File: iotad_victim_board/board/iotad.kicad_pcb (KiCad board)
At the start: 2 copper layers, 27.9 x 27.9 mm, 30 parts, among them P1 CONN_01X10, P2 CONN_01X06, U11 24C16, U2 MAX31820

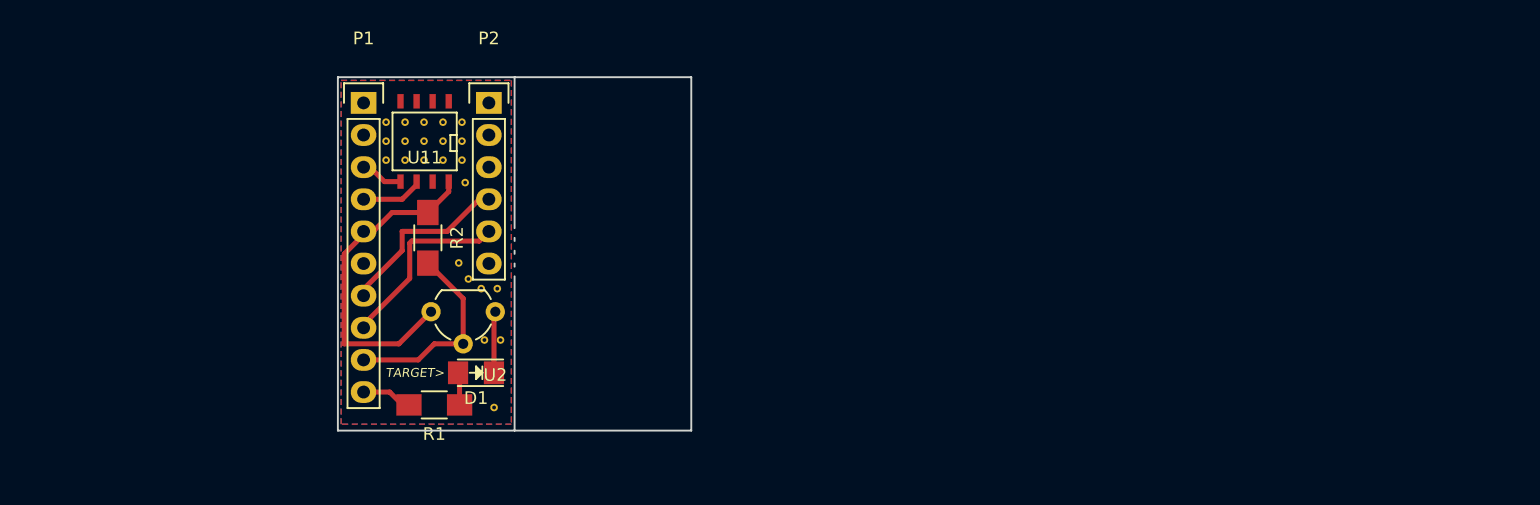
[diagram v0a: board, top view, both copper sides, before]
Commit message: storing
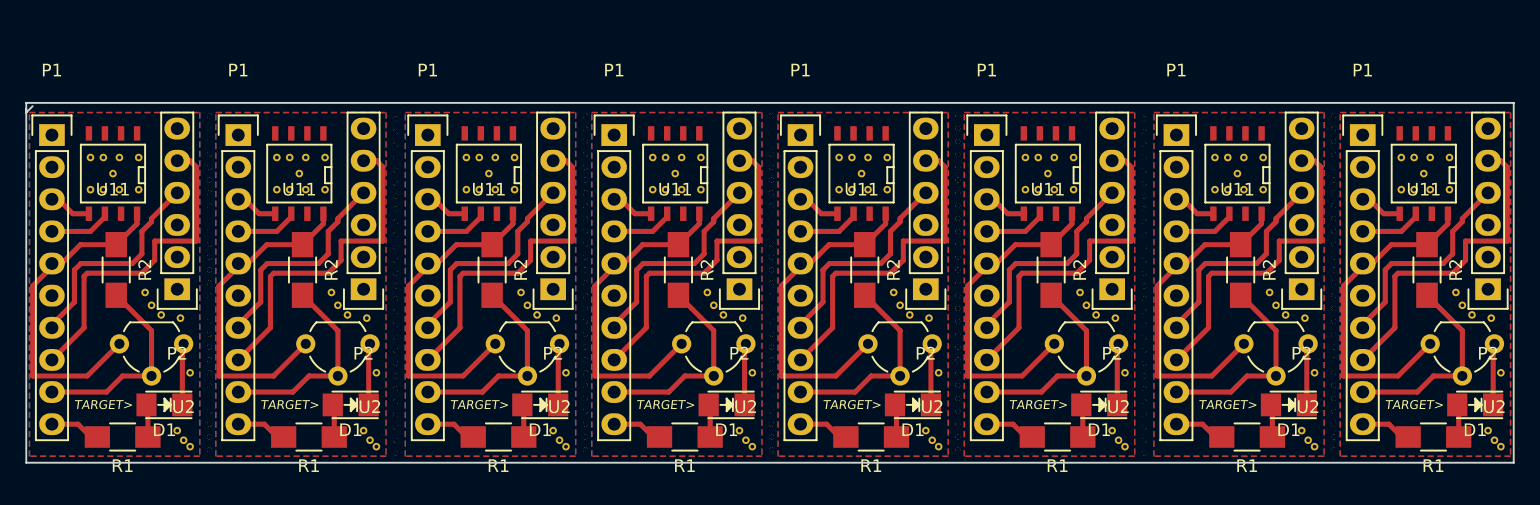
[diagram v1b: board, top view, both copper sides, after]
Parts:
- added D1: LED, LEDs:LED_1206, F.Cu at (182.6, 127.5)
- added D1: LED, LEDs:LED_1206, F.Cu at (197.4, 127.5)
- added D1: LED, LEDs:LED_1206, F.Cu at (227.1, 127.5)
- added D1: LED, LEDs:LED_1206, F.Cu at (212.3, 127.5)
- added D1: LED, LEDs:LED_1206, F.Cu at (153.2, 127.5)
- added D1: LED, LEDs:LED_1206, F.Cu at (167.9, 127.5)
- added D1: LED, LEDs:LED_1206, F.Cu at (138.2, 127.5)
- added P1: CONN_01X10, Pin_Headers:Pin_Header_Straight_1x10, F.Cu at (173.7, 106.2)
- added P1: CONN_01X10, Pin_Headers:Pin_Header_Straight_1x10, F.Cu at (188.5, 106.2)
- added P1: CONN_01X10, Pin_Headers:Pin_Header_Straight_1x10, F.Cu at (218.2, 106.2)
- added P1: CONN_01X10, Pin_Headers:Pin_Header_Straight_1x10, F.Cu at (203.5, 106.2)
- added P1: CONN_01X10, Pin_Headers:Pin_Header_Straight_1x10, F.Cu at (144.3, 106.2)
- added P1: CONN_01X10, Pin_Headers:Pin_Header_Straight_1x10, F.Cu at (159.0, 106.2)
- added P1: CONN_01X10, Pin_Headers:Pin_Header_Straight_1x10, F.Cu at (129.3, 106.2)
- added P2: CONN_01X06, Pin_Headers:Pin_Header_Straight_1x06, F.Cu at (183.6, 118.4)
- added P2: CONN_01X06, Pin_Headers:Pin_Header_Straight_1x06, F.Cu at (198.4, 118.4)
- added P2: CONN_01X06, Pin_Headers:Pin_Header_Straight_1x06, F.Cu at (228.1, 118.4)
- added P2: CONN_01X06, Pin_Headers:Pin_Header_Straight_1x06, F.Cu at (213.4, 118.4)
- added P2: CONN_01X06, Pin_Headers:Pin_Header_Straight_1x06, F.Cu at (154.2, 118.4)
- added P2: CONN_01X06, Pin_Headers:Pin_Header_Straight_1x06, F.Cu at (168.9, 118.4)
- added P2: CONN_01X06, Pin_Headers:Pin_Header_Straight_1x06, F.Cu at (139.2, 118.4)
- added R1: R, Resistors_SMD:R_1206_HandSoldering, F.Cu at (179.3, 130.0)
- added R1: R, Resistors_SMD:R_1206_HandSoldering, F.Cu at (194.1, 130.0)
- added R1: R, Resistors_SMD:R_1206_HandSoldering, F.Cu at (223.8, 130.0)
- added R1: R, Resistors_SMD:R_1206_HandSoldering, F.Cu at (209.0, 130.0)
- added R1: R, Resistors_SMD:R_1206_HandSoldering, F.Cu at (149.9, 130.0)
- added R1: R, Resistors_SMD:R_1206_HandSoldering, F.Cu at (164.6, 130.0)
- added R1: R, Resistors_SMD:R_1206_HandSoldering, F.Cu at (134.9, 130.0)
- added R2: 4.8k, Resistors_SMD:R_1206_HandSoldering, F.Cu at (178.8, 116.8)
- added R2: 4.8k, Resistors_SMD:R_1206_HandSoldering, F.Cu at (193.5, 116.8)
- added R2: 4.8k, Resistors_SMD:R_1206_HandSoldering, F.Cu at (223.3, 116.8)
- added R2: 4.8k, Resistors_SMD:R_1206_HandSoldering, F.Cu at (208.5, 116.8)
- added R2: 4.8k, Resistors_SMD:R_1206_HandSoldering, F.Cu at (149.4, 116.8)
- added R2: 4.8k, Resistors_SMD:R_1206_HandSoldering, F.Cu at (164.1, 116.8)
- added R2: 4.8k, Resistors_SMD:R_1206_HandSoldering, F.Cu at (134.4, 116.8)
- added REF** (x4): DRILL-0.6mm, via-0:DRILL-0.6mm, F.Cu at (186.2, 107.7)
- added REF** (x4): DRILL-0.6mm, via-0:DRILL-0.6mm, F.Cu at (186.2, 104.6)
- added REF** (x4): DRILL-0.6mm, via-0:DRILL-0.6mm, F.Cu at (186.2, 121.9)
- added REF** (x4): DRILL-0.6mm, via-0:DRILL-0.6mm, F.Cu at (186.2, 124.0)
- added REF** (x4): DRILL-0.6mm, via-0:DRILL-0.6mm, F.Cu at (186.2, 122.9)
- added REF** (x4): DRILL-0.6mm, via-0:DRILL-0.6mm, F.Cu at (215.9, 124.0)
- added REF** (x4): DRILL-0.6mm, via-0:DRILL-0.6mm, F.Cu at (215.9, 122.9)
- added REF** (x4): DRILL-0.6mm, via-0:DRILL-0.6mm, F.Cu at (215.9, 121.9)
- added REF** (x4): DRILL-0.6mm, via-0:DRILL-0.6mm, F.Cu at (215.9, 120.9)
- added REF** (x4): DRILL-0.6mm, via-0:DRILL-0.6mm, F.Cu at (186.2, 105.7)
- added REF** (x4): DRILL-0.6mm, via-0:DRILL-0.6mm, F.Cu at (215.9, 126.0)
- added REF** (x4): DRILL-0.6mm, via-0:DRILL-0.6mm, F.Cu at (215.9, 125.0)
- added REF** (x4): DRILL-0.6mm, via-0:DRILL-0.6mm, F.Cu at (215.9, 128.0)
- added REF** (x4): DRILL-0.6mm, via-0:DRILL-0.6mm, F.Cu at (215.9, 127.0)
- added REF** (x4): DRILL-0.6mm, via-0:DRILL-0.6mm, F.Cu at (215.9, 130.0)
- added REF** (x4): DRILL-0.6mm, via-0:DRILL-0.6mm, F.Cu at (215.9, 129.0)
- added REF** (x4): DRILL-0.6mm, via-0:DRILL-0.6mm, F.Cu at (215.9, 131.1)
- added REF** (x4): DRILL-0.6mm, via-0:DRILL-0.6mm, F.Cu at (215.9, 115.8)
- added REF** (x4): DRILL-0.6mm, via-0:DRILL-0.6mm, F.Cu at (215.9, 114.8)
- added REF** (x4): DRILL-0.6mm, via-0:DRILL-0.6mm, F.Cu at (215.9, 113.8)
- added REF** (x4): DRILL-0.6mm, via-0:DRILL-0.6mm, F.Cu at (215.9, 112.8)
- added REF** (x4): DRILL-0.6mm, via-0:DRILL-0.6mm, F.Cu at (215.9, 117.9)
- added REF** (x4): DRILL-0.6mm, via-0:DRILL-0.6mm, F.Cu at (186.2, 109.7)
- added REF** (x4): DRILL-0.6mm, via-0:DRILL-0.6mm, F.Cu at (215.9, 116.8)
- added REF** (x4): DRILL-0.6mm, via-0:DRILL-0.6mm, F.Cu at (215.9, 119.9)
- added REF** (x4): DRILL-0.6mm, via-0:DRILL-0.6mm, F.Cu at (215.9, 118.9)
- added REF** (x4): DRILL-0.6mm, via-0:DRILL-0.6mm, F.Cu at (186.2, 108.7)
- added REF** (x4): DRILL-0.6mm, via-0:DRILL-0.6mm, F.Cu at (215.9, 111.8)
- added REF** (x4): DRILL-0.6mm, via-0:DRILL-0.6mm, F.Cu at (215.9, 110.7)
- added REF** (x4): DRILL-0.6mm, via-0:DRILL-0.6mm, F.Cu at (215.9, 109.7)
- added REF** (x4): DRILL-0.6mm, via-0:DRILL-0.6mm, F.Cu at (215.9, 108.7)
- added REF** (x4): DRILL-0.6mm, via-0:DRILL-0.6mm, F.Cu at (186.2, 106.7)
- added REF** (x4): DRILL-0.6mm, via-0:DRILL-0.6mm, F.Cu at (215.9, 105.7)
- added REF** (x4): DRILL-0.6mm, via-0:DRILL-0.6mm, F.Cu at (215.9, 104.6)
- added REF** (x4): DRILL-0.6mm, via-0:DRILL-0.6mm, F.Cu at (215.9, 107.7)
- added REF** (x4): DRILL-0.6mm, via-0:DRILL-0.6mm, F.Cu at (215.9, 106.7)
- added REF** (x4): DRILL-0.6mm, via-0:DRILL-0.6mm, F.Cu at (200.9, 124.2)
- added REF** (x4): DRILL-0.6mm, via-0:DRILL-0.6mm, F.Cu at (200.9, 123.2)
- added REF** (x4): DRILL-0.6mm, via-0:DRILL-0.6mm, F.Cu at (200.9, 122.2)
- added REF** (x4): DRILL-0.6mm, via-0:DRILL-0.6mm, F.Cu at (200.9, 121.2)
- added REF** (x4): DRILL-0.6mm, via-0:DRILL-0.6mm, F.Cu at (200.9, 126.2)
- added REF** (x4): DRILL-0.6mm, via-0:DRILL-0.6mm, F.Cu at (200.9, 125.2)
- added REF** (x4): DRILL-0.6mm, via-0:DRILL-0.6mm, F.Cu at (200.9, 128.3)
- added REF** (x4): DRILL-0.6mm, via-0:DRILL-0.6mm, F.Cu at (200.9, 127.3)
- added REF** (x4): DRILL-0.6mm, via-0:DRILL-0.6mm, F.Cu at (200.9, 130.3)
- added REF** (x4): DRILL-0.6mm, via-0:DRILL-0.6mm, F.Cu at (186.2, 111.8)
- added REF** (x4): DRILL-0.6mm, via-0:DRILL-0.6mm, F.Cu at (200.9, 129.3)
- added REF** (x4): DRILL-0.6mm, via-0:DRILL-0.6mm, F.Cu at (200.9, 131.3)
- added REF** (x4): DRILL-0.6mm, via-0:DRILL-0.6mm, F.Cu at (186.2, 110.7)
- added REF** (x4): DRILL-0.6mm, via-0:DRILL-0.6mm, F.Cu at (200.9, 116.1)
- added REF** (x4): DRILL-0.6mm, via-0:DRILL-0.6mm, F.Cu at (200.9, 115.1)
- added REF** (x4): DRILL-0.6mm, via-0:DRILL-0.6mm, F.Cu at (200.9, 114.0)
- added REF** (x4): DRILL-0.6mm, via-0:DRILL-0.6mm, F.Cu at (200.9, 113.0)
- added REF** (x4): DRILL-0.6mm, via-0:DRILL-0.6mm, F.Cu at (200.9, 118.1)
- added REF** (x4): DRILL-0.6mm, via-0:DRILL-0.6mm, F.Cu at (200.9, 117.1)
- added REF** (x4): DRILL-0.6mm, via-0:DRILL-0.6mm, F.Cu at (200.9, 120.1)
- added REF** (x4): DRILL-0.6mm, via-0:DRILL-0.6mm, F.Cu at (200.9, 119.1)
- added REF** (x4): DRILL-0.6mm, via-0:DRILL-0.6mm, F.Cu at (200.9, 112.0)
- added REF** (x4): DRILL-0.6mm, via-0:DRILL-0.6mm, F.Cu at (200.9, 111.0)
- added REF** (x4): DRILL-0.6mm, via-0:DRILL-0.6mm, F.Cu at (200.9, 110.0)
- added REF** (x4): DRILL-0.6mm, via-0:DRILL-0.6mm, F.Cu at (200.9, 109.0)
- added REF** (x4): DRILL-0.6mm, via-0:DRILL-0.6mm, F.Cu at (200.9, 105.9)
- added REF** (x4): DRILL-0.6mm, via-0:DRILL-0.6mm, F.Cu at (200.9, 104.9)
- added REF** (x4): DRILL-0.6mm, via-0:DRILL-0.6mm, F.Cu at (200.9, 108.0)
- added REF** (x4): DRILL-0.6mm, via-0:DRILL-0.6mm, F.Cu at (200.9, 106.9)
- added REF** (x4): DRILL-0.6mm, via-0:DRILL-0.6mm, F.Cu at (141.7, 108.0)
- added REF** (x4): DRILL-0.6mm, via-0:DRILL-0.6mm, F.Cu at (141.7, 106.9)
- added REF** (x4): DRILL-0.6mm, via-0:DRILL-0.6mm, F.Cu at (186.2, 119.9)
- added REF** (x4): DRILL-0.6mm, via-0:DRILL-0.6mm, F.Cu at (141.7, 105.9)
- added REF** (x4): DRILL-0.6mm, via-0:DRILL-0.6mm, F.Cu at (141.7, 104.9)
- added REF** (x4): DRILL-0.6mm, via-0:DRILL-0.6mm, F.Cu at (186.2, 118.9)
- added REF** (x4): DRILL-0.6mm, via-0:DRILL-0.6mm, F.Cu at (141.7, 110.0)
- added REF** (x4): DRILL-0.6mm, via-0:DRILL-0.6mm, F.Cu at (141.7, 109.0)
- added REF** (x4): DRILL-0.6mm, via-0:DRILL-0.6mm, F.Cu at (141.7, 112.0)
- added REF** (x4): DRILL-0.6mm, via-0:DRILL-0.6mm, F.Cu at (141.7, 111.0)
- added REF** (x4): DRILL-0.6mm, via-0:DRILL-0.6mm, F.Cu at (141.7, 120.1)
- added REF** (x4): DRILL-0.6mm, via-0:DRILL-0.6mm, F.Cu at (141.7, 119.1)
- added REF** (x4): DRILL-0.6mm, via-0:DRILL-0.6mm, F.Cu at (141.7, 118.1)
- added REF** (x4): DRILL-0.6mm, via-0:DRILL-0.6mm, F.Cu at (141.7, 117.1)
- added REF** (x4): DRILL-0.6mm, via-0:DRILL-0.6mm, F.Cu at (141.7, 114.0)
- added REF** (x4): DRILL-0.6mm, via-0:DRILL-0.6mm, F.Cu at (141.7, 113.0)
- added REF** (x4): DRILL-0.6mm, via-0:DRILL-0.6mm, F.Cu at (141.7, 116.1)
- added REF** (x4): DRILL-0.6mm, via-0:DRILL-0.6mm, F.Cu at (141.7, 115.1)
- added REF** (x4): DRILL-0.6mm, via-0:DRILL-0.6mm, F.Cu at (141.7, 131.3)
- added REF** (x4): DRILL-0.6mm, via-0:DRILL-0.6mm, F.Cu at (141.7, 130.3)
- added REF** (x4): DRILL-0.6mm, via-0:DRILL-0.6mm, F.Cu at (141.7, 129.3)
- added REF** (x4): DRILL-0.6mm, via-0:DRILL-0.6mm, F.Cu at (141.7, 128.3)
- added REF** (x4): DRILL-0.6mm, via-0:DRILL-0.6mm, F.Cu at (141.7, 127.3)
- added REF** (x4): DRILL-0.6mm, via-0:DRILL-0.6mm, F.Cu at (141.7, 126.2)
- added REF** (x4): DRILL-0.6mm, via-0:DRILL-0.6mm, F.Cu at (186.2, 117.9)
- added REF** (x4): DRILL-0.6mm, via-0:DRILL-0.6mm, F.Cu at (141.7, 125.2)
- added REF** (x4): DRILL-0.6mm, via-0:DRILL-0.6mm, F.Cu at (141.7, 122.2)
- added REF** (x4): DRILL-0.6mm, via-0:DRILL-0.6mm, F.Cu at (141.7, 121.2)
- added REF** (x4): DRILL-0.6mm, via-0:DRILL-0.6mm, F.Cu at (186.2, 116.8)
- added REF** (x4): DRILL-0.6mm, via-0:DRILL-0.6mm, F.Cu at (141.7, 124.2)
- added REF** (x4): DRILL-0.6mm, via-0:DRILL-0.6mm, F.Cu at (141.7, 123.2)
- added REF** (x4): DRILL-0.6mm, via-0:DRILL-0.6mm, F.Cu at (171.4, 124.0)
- added REF** (x4): DRILL-0.6mm, via-0:DRILL-0.6mm, F.Cu at (171.4, 122.9)
- added REF** (x4): DRILL-0.6mm, via-0:DRILL-0.6mm, F.Cu at (171.4, 121.9)
- added REF** (x4): DRILL-0.6mm, via-0:DRILL-0.6mm, F.Cu at (171.4, 120.9)
- added REF** (x4): DRILL-0.6mm, via-0:DRILL-0.6mm, F.Cu at (171.4, 126.0)
- added REF** (x4): DRILL-0.6mm, via-0:DRILL-0.6mm, F.Cu at (171.4, 125.0)
- added REF** (x4): DRILL-0.6mm, via-0:DRILL-0.6mm, F.Cu at (171.4, 128.0)
- added REF** (x4): DRILL-0.6mm, via-0:DRILL-0.6mm, F.Cu at (171.4, 127.0)
- added REF** (x4): DRILL-0.6mm, via-0:DRILL-0.6mm, F.Cu at (171.4, 130.0)
- added REF** (x4): DRILL-0.6mm, via-0:DRILL-0.6mm, F.Cu at (171.4, 129.0)
- added REF** (x4): DRILL-0.6mm, via-0:DRILL-0.6mm, F.Cu at (171.4, 131.1)
- added REF** (x4): DRILL-0.6mm, via-0:DRILL-0.6mm, F.Cu at (171.4, 115.8)
- added REF** (x4): DRILL-0.6mm, via-0:DRILL-0.6mm, F.Cu at (171.4, 114.8)
- added REF** (x4): DRILL-0.6mm, via-0:DRILL-0.6mm, F.Cu at (171.4, 113.8)
- added REF** (x4): DRILL-0.6mm, via-0:DRILL-0.6mm, F.Cu at (171.4, 112.8)
- added REF** (x4): DRILL-0.6mm, via-0:DRILL-0.6mm, F.Cu at (186.2, 113.8)
- added REF** (x4): DRILL-0.6mm, via-0:DRILL-0.6mm, F.Cu at (171.4, 117.9)
- added REF** (x4): DRILL-0.6mm, via-0:DRILL-0.6mm, F.Cu at (171.4, 116.8)
- added REF** (x4): DRILL-0.6mm, via-0:DRILL-0.6mm, F.Cu at (186.2, 112.8)
- added REF** (x4): DRILL-0.6mm, via-0:DRILL-0.6mm, F.Cu at (171.4, 119.9)
- added REF** (x4): DRILL-0.6mm, via-0:DRILL-0.6mm, F.Cu at (171.4, 118.9)
- added REF** (x4): DRILL-0.6mm, via-0:DRILL-0.6mm, F.Cu at (171.4, 111.8)
- added REF** (x4): DRILL-0.6mm, via-0:DRILL-0.6mm, F.Cu at (171.4, 110.7)
- added REF** (x4): DRILL-0.6mm, via-0:DRILL-0.6mm, F.Cu at (171.4, 109.7)
- added REF** (x4): DRILL-0.6mm, via-0:DRILL-0.6mm, F.Cu at (171.4, 108.7)
- added REF** (x4): DRILL-0.6mm, via-0:DRILL-0.6mm, F.Cu at (171.4, 105.7)
- added REF** (x4): DRILL-0.6mm, via-0:DRILL-0.6mm, F.Cu at (171.4, 104.6)
- added REF** (x4): DRILL-0.6mm, via-0:DRILL-0.6mm, F.Cu at (171.4, 107.7)
- added REF** (x4): DRILL-0.6mm, via-0:DRILL-0.6mm, F.Cu at (171.4, 106.7)
- added REF** (x4): DRILL-0.6mm, via-0:DRILL-0.6mm, F.Cu at (156.7, 107.7)
- added REF** (x4): DRILL-0.6mm, via-0:DRILL-0.6mm, F.Cu at (156.7, 106.7)
- added REF** (x4): DRILL-0.6mm, via-0:DRILL-0.6mm, F.Cu at (156.7, 105.7)
- added REF** (x4): DRILL-0.6mm, via-0:DRILL-0.6mm, F.Cu at (156.7, 104.6)
- added REF** (x4): DRILL-0.6mm, via-0:DRILL-0.6mm, F.Cu at (156.7, 109.7)
- added REF** (x4): DRILL-0.6mm, via-0:DRILL-0.6mm, F.Cu at (156.7, 108.7)
- added REF** (x4): DRILL-0.6mm, via-0:DRILL-0.6mm, F.Cu at (156.7, 111.8)
- added REF** (x4): DRILL-0.6mm, via-0:DRILL-0.6mm, F.Cu at (156.7, 110.7)
- added REF** (x4): DRILL-0.6mm, via-0:DRILL-0.6mm, F.Cu at (186.2, 115.8)
- added REF** (x4): DRILL-0.6mm, via-0:DRILL-0.6mm, F.Cu at (156.7, 119.9)
- added REF** (x4): DRILL-0.6mm, via-0:DRILL-0.6mm, F.Cu at (156.7, 118.9)
- added REF** (x4): DRILL-0.6mm, via-0:DRILL-0.6mm, F.Cu at (186.2, 114.8)
- added REF** (x4): DRILL-0.6mm, via-0:DRILL-0.6mm, F.Cu at (156.7, 117.9)
- added REF** (x4): DRILL-0.6mm, via-0:DRILL-0.6mm, F.Cu at (156.7, 116.8)
- added REF** (x4): DRILL-0.6mm, via-0:DRILL-0.6mm, F.Cu at (156.7, 113.8)
- added REF** (x4): DRILL-0.6mm, via-0:DRILL-0.6mm, F.Cu at (156.7, 112.8)
- added REF** (x4): DRILL-0.6mm, via-0:DRILL-0.6mm, F.Cu at (156.7, 115.8)
- added REF** (x4): DRILL-0.6mm, via-0:DRILL-0.6mm, F.Cu at (156.7, 114.8)
- added REF** (x4): DRILL-0.6mm, via-0:DRILL-0.6mm, F.Cu at (156.7, 131.1)
- added REF** (x4): DRILL-0.6mm, via-0:DRILL-0.6mm, F.Cu at (156.7, 130.0)
- added REF** (x4): DRILL-0.6mm, via-0:DRILL-0.6mm, F.Cu at (156.7, 129.0)
- added REF** (x4): DRILL-0.6mm, via-0:DRILL-0.6mm, F.Cu at (156.7, 128.0)
- added REF** (x4): DRILL-0.6mm, via-0:DRILL-0.6mm, F.Cu at (156.7, 127.0)
- added REF** (x4): DRILL-0.6mm, via-0:DRILL-0.6mm, F.Cu at (156.7, 126.0)
- added REF** (x4): DRILL-0.6mm, via-0:DRILL-0.6mm, F.Cu at (156.7, 125.0)
- added REF** (x4): DRILL-0.6mm, via-0:DRILL-0.6mm, F.Cu at (156.7, 121.9)
- added REF** (x4): DRILL-0.6mm, via-0:DRILL-0.6mm, F.Cu at (156.7, 120.9)
- added REF** (x4): DRILL-0.6mm, via-0:DRILL-0.6mm, F.Cu at (156.7, 124.0)
- added REF** (x4): DRILL-0.6mm, via-0:DRILL-0.6mm, F.Cu at (156.7, 122.9)
- added REF** (x4): DRILL-0.6mm, via-0:DRILL-0.6mm, F.Cu at (127.0, 124.0)
- added REF** (x4): DRILL-0.6mm, via-0:DRILL-0.6mm, F.Cu at (186.2, 131.1)
- added REF** (x4): DRILL-0.6mm, via-0:DRILL-0.6mm, F.Cu at (127.0, 122.9)
- added REF** (x4): DRILL-0.6mm, via-0:DRILL-0.6mm, F.Cu at (127.0, 121.9)
- added REF** (x4): DRILL-0.6mm, via-0:DRILL-0.6mm, F.Cu at (127.0, 120.9)
- added REF** (x4): DRILL-0.6mm, via-0:DRILL-0.6mm, F.Cu at (127.0, 126.0)
- added REF** (x4): DRILL-0.6mm, via-0:DRILL-0.6mm, F.Cu at (127.0, 125.0)
- added REF** (x4): DRILL-0.6mm, via-0:DRILL-0.6mm, F.Cu at (127.0, 128.0)
- added REF** (x4): DRILL-0.6mm, via-0:DRILL-0.6mm, F.Cu at (127.0, 127.0)
- added REF** (x4): DRILL-0.6mm, via-0:DRILL-0.6mm, F.Cu at (127.0, 130.0)
- added REF** (x4): DRILL-0.6mm, via-0:DRILL-0.6mm, F.Cu at (127.0, 129.0)
- added REF** (x4): DRILL-0.6mm, via-0:DRILL-0.6mm, F.Cu at (127.0, 131.1)
- added REF** (x4): DRILL-0.6mm, via-0:DRILL-0.6mm, F.Cu at (186.2, 130.0)
- added REF** (x4): DRILL-0.6mm, via-0:DRILL-0.6mm, F.Cu at (127.0, 115.8)
- added REF** (x4): DRILL-0.6mm, via-0:DRILL-0.6mm, F.Cu at (127.0, 114.8)
- added REF** (x4): DRILL-0.6mm, via-0:DRILL-0.6mm, F.Cu at (186.2, 129.0)
- added REF** (x4): DRILL-0.6mm, via-0:DRILL-0.6mm, F.Cu at (127.0, 113.8)
- added REF** (x4): DRILL-0.6mm, via-0:DRILL-0.6mm, F.Cu at (127.0, 112.8)
- added REF** (x4): DRILL-0.6mm, via-0:DRILL-0.6mm, F.Cu at (127.0, 117.9)
- added REF** (x4): DRILL-0.6mm, via-0:DRILL-0.6mm, F.Cu at (127.0, 116.8)
- added REF** (x4): DRILL-0.6mm, via-0:DRILL-0.6mm, F.Cu at (127.0, 119.9)
- added REF** (x4): DRILL-0.6mm, via-0:DRILL-0.6mm, F.Cu at (127.0, 118.9)
- added REF** (x4): DRILL-0.6mm, via-0:DRILL-0.6mm, F.Cu at (127.0, 111.8)
- added REF** (x4): DRILL-0.6mm, via-0:DRILL-0.6mm, F.Cu at (127.0, 110.7)
- added REF** (x4): DRILL-0.6mm, via-0:DRILL-0.6mm, F.Cu at (127.0, 109.7)
- added REF** (x4): DRILL-0.6mm, via-0:DRILL-0.6mm, F.Cu at (127.0, 108.7)
- added REF** (x4): DRILL-0.6mm, via-0:DRILL-0.6mm, F.Cu at (127.0, 105.7)
- added REF** (x4): DRILL-0.6mm, via-0:DRILL-0.6mm, F.Cu at (127.0, 104.6)
- added REF** (x4): DRILL-0.6mm, via-0:DRILL-0.6mm, F.Cu at (127.0, 107.7)
- added REF** (x4): DRILL-0.6mm, via-0:DRILL-0.6mm, F.Cu at (127.0, 106.7)
- added REF** (x4): DRILL-0.6mm, via-0:DRILL-0.6mm, F.Cu at (186.2, 128.0)
- added REF** (x4): DRILL-0.6mm, via-0:DRILL-0.6mm, F.Cu at (186.2, 127.0)
- added REF** (x4): DRILL-0.6mm, via-0:DRILL-0.6mm, F.Cu at (186.2, 126.0)
- added REF** (x4): DRILL-0.6mm, via-0:DRILL-0.6mm, F.Cu at (186.2, 125.0)
- added REF** (x4): DRILL-0.6mm, via-0:DRILL-0.6mm, F.Cu at (186.2, 120.9)
- added REF**1111: VIA-0.6mm, via-0:VIA-0.6mm, F.Cu at (175.5, 107.7)
- added REF**1111: VIA-0.6mm, via-0:VIA-0.6mm, F.Cu at (190.2, 107.7)
- added REF**1111: VIA-0.6mm, via-0:VIA-0.6mm, F.Cu at (220.0, 107.7)
- added REF**1111: VIA-0.6mm, via-0:VIA-0.6mm, F.Cu at (205.2, 107.7)
- added REF**1111: VIA-0.6mm, via-0:VIA-0.6mm, F.Cu at (146.1, 107.7)
- added REF**1111: VIA-0.6mm, via-0:VIA-0.6mm, F.Cu at (160.8, 107.7)
- added REF**1111: VIA-0.6mm, via-0:VIA-0.6mm, F.Cu at (131.1, 107.7)
- added REF**1112: VIA-0.6mm, via-0:VIA-0.6mm, F.Cu at (175.5, 109.2)
- added REF**1112: VIA-0.6mm, via-0:VIA-0.6mm, F.Cu at (190.2, 109.2)
- added REF**1112: VIA-0.6mm, via-0:VIA-0.6mm, F.Cu at (220.0, 109.2)
- added REF**1112: VIA-0.6mm, via-0:VIA-0.6mm, F.Cu at (205.2, 109.2)
- added REF**1112: VIA-0.6mm, via-0:VIA-0.6mm, F.Cu at (146.1, 109.2)
- added REF**1112: VIA-0.6mm, via-0:VIA-0.6mm, F.Cu at (160.8, 109.2)
- added REF**1112: VIA-0.6mm, via-0:VIA-0.6mm, F.Cu at (131.1, 109.2)
- added REF**1113: VIA-0.6mm, via-0:VIA-0.6mm, F.Cu at (175.5, 110.7)
- added REF**1113: VIA-0.6mm, via-0:VIA-0.6mm, F.Cu at (190.2, 110.7)
- added REF**1113: VIA-0.6mm, via-0:VIA-0.6mm, F.Cu at (220.0, 110.7)
- added REF**1113: VIA-0.6mm, via-0:VIA-0.6mm, F.Cu at (205.2, 110.7)
- added REF**1113: VIA-0.6mm, via-0:VIA-0.6mm, F.Cu at (146.1, 110.7)
- added REF**1113: VIA-0.6mm, via-0:VIA-0.6mm, F.Cu at (160.8, 110.7)
- added REF**1113: VIA-0.6mm, via-0:VIA-0.6mm, F.Cu at (131.1, 110.7)
- added REF**1121: VIA-0.6mm, via-0:VIA-0.6mm, F.Cu at (183.6, 129.5)
- added REF**1121: VIA-0.6mm, via-0:VIA-0.6mm, F.Cu at (198.4, 129.5)
- added REF**1121: VIA-0.6mm, via-0:VIA-0.6mm, F.Cu at (228.1, 129.5)
- added REF**1121: VIA-0.6mm, via-0:VIA-0.6mm, F.Cu at (213.4, 129.5)
- added REF**1121: VIA-0.6mm, via-0:VIA-0.6mm, F.Cu at (154.2, 129.5)
- added REF**1121: VIA-0.6mm, via-0:VIA-0.6mm, F.Cu at (168.9, 129.5)
- added REF**1121: VIA-0.6mm, via-0:VIA-0.6mm, F.Cu at (139.2, 129.5)
- added REF**1122: VIA-0.6mm, via-0:VIA-0.6mm, F.Cu at (177.0, 109.2)
- added REF**1122: VIA-0.6mm, via-0:VIA-0.6mm, F.Cu at (191.7, 109.2)
- added REF**1122: VIA-0.6mm, via-0:VIA-0.6mm, F.Cu at (221.5, 109.2)
- added REF**1122: VIA-0.6mm, via-0:VIA-0.6mm, F.Cu at (206.7, 109.2)
- added REF**1122: VIA-0.6mm, via-0:VIA-0.6mm, F.Cu at (147.6, 109.2)
- added REF**1122: VIA-0.6mm, via-0:VIA-0.6mm, F.Cu at (162.3, 109.2)
- added REF**1122: VIA-0.6mm, via-0:VIA-0.6mm, F.Cu at (132.6, 109.2)
- added REF**1123: VIA-0.6mm, via-0:VIA-0.6mm, F.Cu at (177.0, 110.7)
- added REF**1123: VIA-0.6mm, via-0:VIA-0.6mm, F.Cu at (191.7, 110.7)
- added REF**1123: VIA-0.6mm, via-0:VIA-0.6mm, F.Cu at (221.5, 110.7)
- added REF**1123: VIA-0.6mm, via-0:VIA-0.6mm, F.Cu at (206.7, 110.7)
- added REF**1123: VIA-0.6mm, via-0:VIA-0.6mm, F.Cu at (147.6, 110.7)
- added REF**1123: VIA-0.6mm, via-0:VIA-0.6mm, F.Cu at (162.3, 110.7)
- added REF**1123: VIA-0.6mm, via-0:VIA-0.6mm, F.Cu at (132.6, 110.7)
- added REF**1131: VIA-0.6mm, via-0:VIA-0.6mm, F.Cu at (180.6, 110.5)
- added REF**1131: VIA-0.6mm, via-0:VIA-0.6mm, F.Cu at (195.3, 110.5)
- added REF**1131: VIA-0.6mm, via-0:VIA-0.6mm, F.Cu at (225.0, 110.5)
- added REF**1131: VIA-0.6mm, via-0:VIA-0.6mm, F.Cu at (210.3, 110.5)
- added REF**1131: VIA-0.6mm, via-0:VIA-0.6mm, F.Cu at (151.1, 110.5)
- added REF**1131: VIA-0.6mm, via-0:VIA-0.6mm, F.Cu at (165.9, 110.5)
- added REF**1131: VIA-0.6mm, via-0:VIA-0.6mm, F.Cu at (136.1, 110.5)
- added REF**1132: VIA-0.6mm, via-0:VIA-0.6mm, F.Cu at (179.1, 110.5)
- added REF**1132: VIA-0.6mm, via-0:VIA-0.6mm, F.Cu at (193.8, 110.5)
- added REF**1132: VIA-0.6mm, via-0:VIA-0.6mm, F.Cu at (223.5, 110.5)
- added REF**1132: VIA-0.6mm, via-0:VIA-0.6mm, F.Cu at (208.8, 110.5)
- added REF**1132: VIA-0.6mm, via-0:VIA-0.6mm, F.Cu at (149.6, 110.5)
- added REF**1132: VIA-0.6mm, via-0:VIA-0.6mm, F.Cu at (164.3, 110.5)
- added REF**1132: VIA-0.6mm, via-0:VIA-0.6mm, F.Cu at (134.6, 110.5)
- added REF**1133: VIA-0.6mm, via-0:VIA-0.6mm, F.Cu at (180.6, 108.0)
- added REF**1133: VIA-0.6mm, via-0:VIA-0.6mm, F.Cu at (195.3, 108.0)
- added REF**1133: VIA-0.6mm, via-0:VIA-0.6mm, F.Cu at (225.0, 108.0)
- added REF**1133: VIA-0.6mm, via-0:VIA-0.6mm, F.Cu at (210.3, 108.0)
- added REF**1133: VIA-0.6mm, via-0:VIA-0.6mm, F.Cu at (151.1, 108.0)
- added REF**1133: VIA-0.6mm, via-0:VIA-0.6mm, F.Cu at (165.9, 108.0)
- added REF**1133: VIA-0.6mm, via-0:VIA-0.6mm, F.Cu at (136.1, 108.0)
- added REF**1141: VIA-0.6mm, via-0:VIA-0.6mm, F.Cu at (177.8, 108.0)
- added REF**1141: VIA-0.6mm, via-0:VIA-0.6mm, F.Cu at (192.5, 108.0)
- added REF**1141: VIA-0.6mm, via-0:VIA-0.6mm, F.Cu at (222.2, 108.0)
- added REF**1141: VIA-0.6mm, via-0:VIA-0.6mm, F.Cu at (207.5, 108.0)
- added REF**1141: VIA-0.6mm, via-0:VIA-0.6mm, F.Cu at (148.3, 108.0)
- added REF**1141: VIA-0.6mm, via-0:VIA-0.6mm, F.Cu at (163.1, 108.0)
- added REF**1141: VIA-0.6mm, via-0:VIA-0.6mm, F.Cu at (133.3, 108.0)
- added REF**1142: VIA-0.6mm, via-0:VIA-0.6mm, F.Cu at (177.8, 110.5)
- added REF**1142: VIA-0.6mm, via-0:VIA-0.6mm, F.Cu at (192.5, 110.5)
- added REF**1142: VIA-0.6mm, via-0:VIA-0.6mm, F.Cu at (222.2, 110.5)
- added REF**1142: VIA-0.6mm, via-0:VIA-0.6mm, F.Cu at (207.5, 110.5)
- added REF**1142: VIA-0.6mm, via-0:VIA-0.6mm, F.Cu at (148.3, 110.5)
- added REF**1142: VIA-0.6mm, via-0:VIA-0.6mm, F.Cu at (163.1, 110.5)
- added REF**1142: VIA-0.6mm, via-0:VIA-0.6mm, F.Cu at (133.3, 110.5)
- added REF**1143: VIA-0.6mm, via-0:VIA-0.6mm, F.Cu at (178.6, 109.2)
- added REF**1143: VIA-0.6mm, via-0:VIA-0.6mm, F.Cu at (193.3, 109.2)
- added REF**1143: VIA-0.6mm, via-0:VIA-0.6mm, F.Cu at (223.0, 109.2)
- added REF**1143: VIA-0.6mm, via-0:VIA-0.6mm, F.Cu at (208.3, 109.2)
- added REF**1143: VIA-0.6mm, via-0:VIA-0.6mm, F.Cu at (149.1, 109.2)
- added REF**1143: VIA-0.6mm, via-0:VIA-0.6mm, F.Cu at (163.8, 109.2)
- added REF**1143: VIA-0.6mm, via-0:VIA-0.6mm, F.Cu at (134.1, 109.2)
- added REF**1151: VIA-0.6mm, via-0:VIA-0.6mm, F.Cu at (176.8, 108.0)
- added REF**1151: VIA-0.6mm, via-0:VIA-0.6mm, F.Cu at (191.5, 108.0)
- added REF**1151: VIA-0.6mm, via-0:VIA-0.6mm, F.Cu at (221.2, 108.0)
- added REF**1151: VIA-0.6mm, via-0:VIA-0.6mm, F.Cu at (206.5, 108.0)
- added REF**1151: VIA-0.6mm, via-0:VIA-0.6mm, F.Cu at (147.3, 108.0)
- added REF**1151: VIA-0.6mm, via-0:VIA-0.6mm, F.Cu at (162.1, 108.0)
- added REF**1151: VIA-0.6mm, via-0:VIA-0.6mm, F.Cu at (132.3, 108.0)
- added REF**1152: VIA-0.6mm, via-0:VIA-0.6mm, F.Cu at (179.1, 108.0)
- added REF**1152: VIA-0.6mm, via-0:VIA-0.6mm, F.Cu at (193.8, 108.0)
- added REF**1152: VIA-0.6mm, via-0:VIA-0.6mm, F.Cu at (223.5, 108.0)
- added REF**1152: VIA-0.6mm, via-0:VIA-0.6mm, F.Cu at (208.8, 108.0)
- added REF**1152: VIA-0.6mm, via-0:VIA-0.6mm, F.Cu at (149.6, 108.0)
- added REF**1152: VIA-0.6mm, via-0:VIA-0.6mm, F.Cu at (164.3, 108.0)
- added REF**1152: VIA-0.6mm, via-0:VIA-0.6mm, F.Cu at (134.6, 108.0)
- added REF**1153: VIA-0.6mm, via-0:VIA-0.6mm, F.Cu at (184.7, 130.8)
- added REF**1153: VIA-0.6mm, via-0:VIA-0.6mm, F.Cu at (197.1, 120.4)
- added REF**1153: VIA-0.6mm, via-0:VIA-0.6mm, F.Cu at (198.9, 130.3)
- added REF**1153: VIA-0.6mm, via-0:VIA-0.6mm, F.Cu at (198.6, 120.7)
- added REF**1153: VIA-0.6mm, via-0:VIA-0.6mm, F.Cu at (196.3, 119.6)
- added REF**1153: VIA-0.6mm, via-0:VIA-0.6mm, F.Cu at (199.4, 125.0)
- added REF**1153: VIA-0.6mm, via-0:VIA-0.6mm, F.Cu at (191.5, 110.5)
- added REF**1153: VIA-0.6mm, via-0:VIA-0.6mm, F.Cu at (195.8, 118.6)
- added REF**1153: VIA-0.6mm, via-0:VIA-0.6mm, F.Cu at (196.5, 112.5)
- added REF**1153: VIA-0.6mm, via-0:VIA-0.6mm, F.Cu at (199.4, 130.8)
- added REF**1153: VIA-0.6mm, via-0:VIA-0.6mm, F.Cu at (229.1, 130.8)
- added REF**1153: VIA-0.6mm, via-0:VIA-0.6mm, F.Cu at (181.8, 112.5)
- added REF**1153: VIA-0.6mm, via-0:VIA-0.6mm, F.Cu at (226.2, 112.5)
- added REF**1153: VIA-0.6mm, via-0:VIA-0.6mm, F.Cu at (225.6, 118.6)
- added REF**1153: VIA-0.6mm, via-0:VIA-0.6mm, F.Cu at (221.2, 110.5)
- added REF**1153: VIA-0.6mm, via-0:VIA-0.6mm, F.Cu at (229.1, 125.0)
- added REF**1153: VIA-0.6mm, via-0:VIA-0.6mm, F.Cu at (226.1, 119.6)
- added REF**1153: VIA-0.6mm, via-0:VIA-0.6mm, F.Cu at (228.3, 120.7)
- added REF**1153: VIA-0.6mm, via-0:VIA-0.6mm, F.Cu at (228.6, 130.3)
- added REF**1153: VIA-0.6mm, via-0:VIA-0.6mm, F.Cu at (226.8, 120.4)
- added REF**1153: VIA-0.6mm, via-0:VIA-0.6mm, F.Cu at (212.1, 120.4)
- added REF**1153: VIA-0.6mm, via-0:VIA-0.6mm, F.Cu at (213.9, 130.3)
- added REF**1153: VIA-0.6mm, via-0:VIA-0.6mm, F.Cu at (181.1, 118.6)
- added REF**1153: VIA-0.6mm, via-0:VIA-0.6mm, F.Cu at (213.6, 120.7)
- added REF**1153: VIA-0.6mm, via-0:VIA-0.6mm, F.Cu at (211.3, 119.6)
- added REF**1153: VIA-0.6mm, via-0:VIA-0.6mm, F.Cu at (214.4, 125.0)
- added REF**1153: VIA-0.6mm, via-0:VIA-0.6mm, F.Cu at (206.5, 110.5)
- added REF**1153: VIA-0.6mm, via-0:VIA-0.6mm, F.Cu at (210.8, 118.6)
- added REF**1153: VIA-0.6mm, via-0:VIA-0.6mm, F.Cu at (211.5, 112.5)
- added REF**1153: VIA-0.6mm, via-0:VIA-0.6mm, F.Cu at (214.4, 130.8)
- added REF**1153: VIA-0.6mm, via-0:VIA-0.6mm, F.Cu at (155.2, 130.8)
- added REF**1153: VIA-0.6mm, via-0:VIA-0.6mm, F.Cu at (152.3, 112.5)
- added REF**1153: VIA-0.6mm, via-0:VIA-0.6mm, F.Cu at (151.6, 118.6)
- added REF**1153: VIA-0.6mm, via-0:VIA-0.6mm, F.Cu at (176.8, 110.5)
- added REF**1153: VIA-0.6mm, via-0:VIA-0.6mm, F.Cu at (147.3, 110.5)
- added REF**1153: VIA-0.6mm, via-0:VIA-0.6mm, F.Cu at (155.2, 125.0)
- added REF**1153: VIA-0.6mm, via-0:VIA-0.6mm, F.Cu at (152.1, 119.6)
- added REF**1153: VIA-0.6mm, via-0:VIA-0.6mm, F.Cu at (154.4, 120.7)
- added REF**1153: VIA-0.6mm, via-0:VIA-0.6mm, F.Cu at (154.7, 130.3)
- added REF**1153: VIA-0.6mm, via-0:VIA-0.6mm, F.Cu at (152.9, 120.4)
- added REF**1153: VIA-0.6mm, via-0:VIA-0.6mm, F.Cu at (167.6, 120.4)
- added REF**1153: VIA-0.6mm, via-0:VIA-0.6mm, F.Cu at (169.4, 130.3)
- added REF**1153: VIA-0.6mm, via-0:VIA-0.6mm, F.Cu at (169.2, 120.7)
- added REF**1153: VIA-0.6mm, via-0:VIA-0.6mm, F.Cu at (166.9, 119.6)
- added REF**1153: VIA-0.6mm, via-0:VIA-0.6mm, F.Cu at (184.7, 125.0)
- added REF**1153: VIA-0.6mm, via-0:VIA-0.6mm, F.Cu at (169.9, 125.0)
- added REF**1153: VIA-0.6mm, via-0:VIA-0.6mm, F.Cu at (162.1, 110.5)
- added REF**1153: VIA-0.6mm, via-0:VIA-0.6mm, F.Cu at (166.4, 118.6)
- added REF**1153: VIA-0.6mm, via-0:VIA-0.6mm, F.Cu at (167.0, 112.5)
- added REF**1153: VIA-0.6mm, via-0:VIA-0.6mm, F.Cu at (169.9, 130.8)
- added REF**1153: VIA-0.6mm, via-0:VIA-0.6mm, F.Cu at (140.2, 130.8)
- added REF**1153: VIA-0.6mm, via-0:VIA-0.6mm, F.Cu at (137.3, 112.5)
- added REF**1153: VIA-0.6mm, via-0:VIA-0.6mm, F.Cu at (136.7, 118.6)
- added REF**1153: VIA-0.6mm, via-0:VIA-0.6mm, F.Cu at (132.3, 110.5)
- added REF**1153: VIA-0.6mm, via-0:VIA-0.6mm, F.Cu at (140.2, 125.0)
- added REF**1153: VIA-0.6mm, via-0:VIA-0.6mm, F.Cu at (181.6, 119.6)
- added REF**1153: VIA-0.6mm, via-0:VIA-0.6mm, F.Cu at (137.2, 119.6)
- added REF**1153: VIA-0.6mm, via-0:VIA-0.6mm, F.Cu at (139.4, 120.7)
- added REF**1153: VIA-0.6mm, via-0:VIA-0.6mm, F.Cu at (139.7, 130.3)
- added REF**1153: VIA-0.6mm, via-0:VIA-0.6mm, F.Cu at (137.9, 120.4)
- added REF**1153: VIA-0.6mm, via-0:VIA-0.6mm, F.Cu at (183.9, 120.7)
- added REF**1153: VIA-0.6mm, via-0:VIA-0.6mm, F.Cu at (184.2, 130.3)
- added REF**1153: VIA-0.6mm, via-0:VIA-0.6mm, F.Cu at (182.4, 120.4)
- added U11: 24C16, SMD_Packages:SOIC-8-N, F.Cu at (178.6, 109.2)
- added U11: 24C16, SMD_Packages:SOIC-8-N, F.Cu at (193.3, 109.2)
- added U11: 24C16, SMD_Packages:SOIC-8-N, F.Cu at (223.0, 109.2)
- added U11: 24C16, SMD_Packages:SOIC-8-N, F.Cu at (208.3, 109.2)
- added U11: 24C16, SMD_Packages:SOIC-8-N, F.Cu at (149.1, 109.2)
- added U11: 24C16, SMD_Packages:SOIC-8-N, F.Cu at (163.8, 109.2)
- added U11: 24C16, SMD_Packages:SOIC-8-N, F.Cu at (134.1, 109.2)
- added U2: MAX31820, TO_SOT_Packages_THT:TO-92_Molded_Wide, F.Cu at (184.2, 122.7)
- added U2: MAX31820, TO_SOT_Packages_THT:TO-92_Molded_Wide, F.Cu at (198.9, 122.7)
- added U2: MAX31820, TO_SOT_Packages_THT:TO-92_Molded_Wide, F.Cu at (228.6, 122.7)
- added U2: MAX31820, TO_SOT_Packages_THT:TO-92_Molded_Wide, F.Cu at (213.9, 122.7)
- added U2: MAX31820, TO_SOT_Packages_THT:TO-92_Molded_Wide, F.Cu at (154.7, 122.7)
- added U2: MAX31820, TO_SOT_Packages_THT:TO-92_Molded_Wide, F.Cu at (169.4, 122.7)
- added U2: MAX31820, TO_SOT_Packages_THT:TO-92_Molded_Wide, F.Cu at (139.7, 122.7)
- moved REF**1153 31.2 mm to (125.5, 130.8)
- moved REF**1153 30.7 mm to (117.6, 110.5)
- moved REF**1121 30.3 mm to (124.5, 129.5)
- moved REF**1151 29.5 mm to (117.6, 108.0)
- moved P2 28.7 mm to (124.5, 118.4), turned to 180 degrees
- moved REF**1153 27.3 mm to (123.2, 120.4)
- moved REF**1142 27.1 mm to (118.6, 110.5)
- moved REF**1152 27.1 mm to (119.9, 108.0)
- moved REF**1141 27.0 mm to (118.6, 108.0)
- moved REF**1143 26.1 mm to (119.4, 109.2)
- moved REF**1153 26.1 mm to (122.4, 119.6)
- moved REF**1153 25.4 mm to (124.7, 120.7)
- moved REF**1153 25.2 mm to (125.5, 125.0)
- moved REF**1153 25.1 mm to (125.0, 130.3)
- moved REF**1153 24.9 mm to (121.9, 118.6)
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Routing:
- net TX: track 14.8 -> 211.4 mm
- net VCC: track 26.3 -> 210.1 mm
- net RX: track 14.3 -> 141.3 mm
- net DATA: track 15.9 -> 127.5 mm
- net SCL: track 4.92 -> 39.3 mm
- net GND: track 4.87 -> 39.0 mm
- net Net-(P1-Pad10): track 4.22 -> 33.8 mm
- net SDA: track 3.39 -> 27.2 mm
- net Net-(D1-Pad2): track 2.59 -> 20.7 mm
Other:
- board size 27.9 x 27.9 mm -> 117.6 x 28.4 mm
- board text added: "IoTAD v1.2.1 15/03/2016 JGV"
- board text removed: "IoTAD v1.2 24/02/2016 JGV"
